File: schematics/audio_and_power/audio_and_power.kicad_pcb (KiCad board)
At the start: 2 copper layers, 85.5 x 88.5 mm, 29 parts, among them J5 Conn_01x03, J6 Conn_01x06, SW1 SW_SPST, SW4 SW_Push, SW5 SW_Push, U2 ESP32-WROOM-32E, U6 MCP4822, U7 PAM8302AAS, U8 LM1117T-3.3

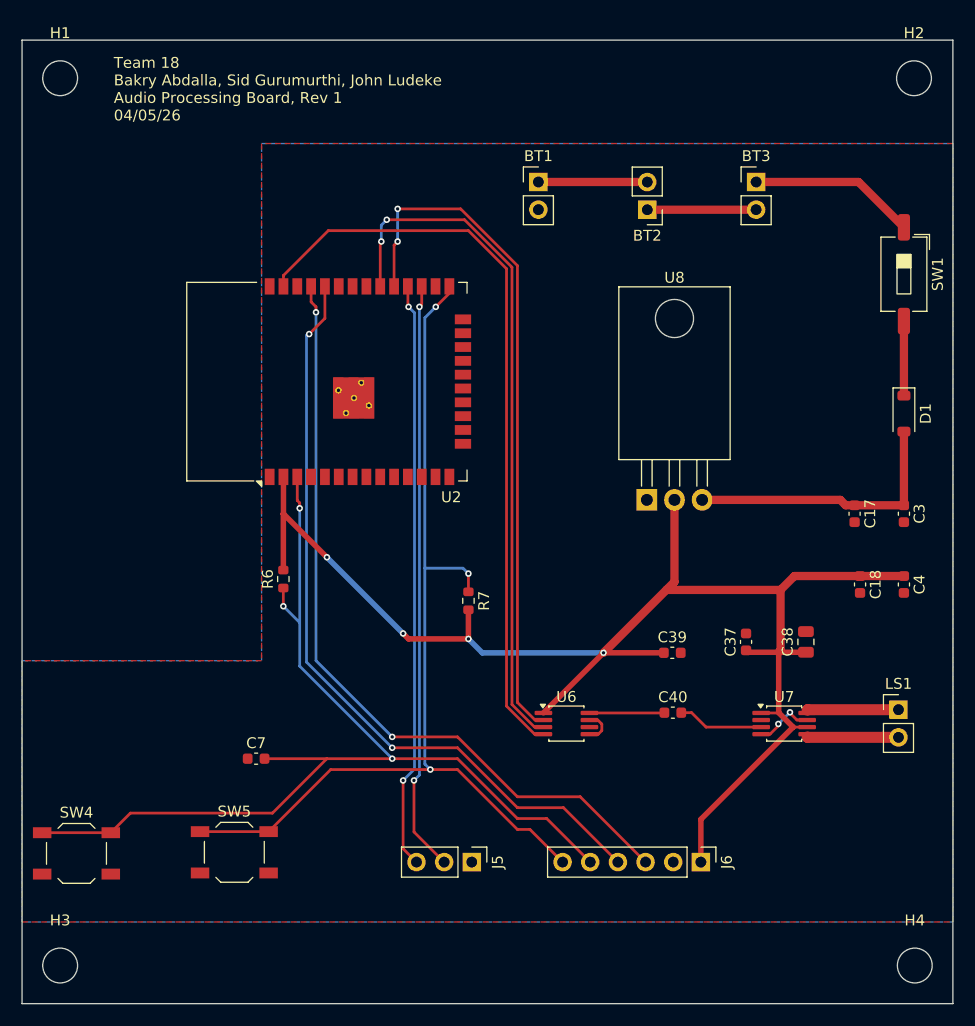
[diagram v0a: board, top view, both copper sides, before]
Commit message: few updates to random things
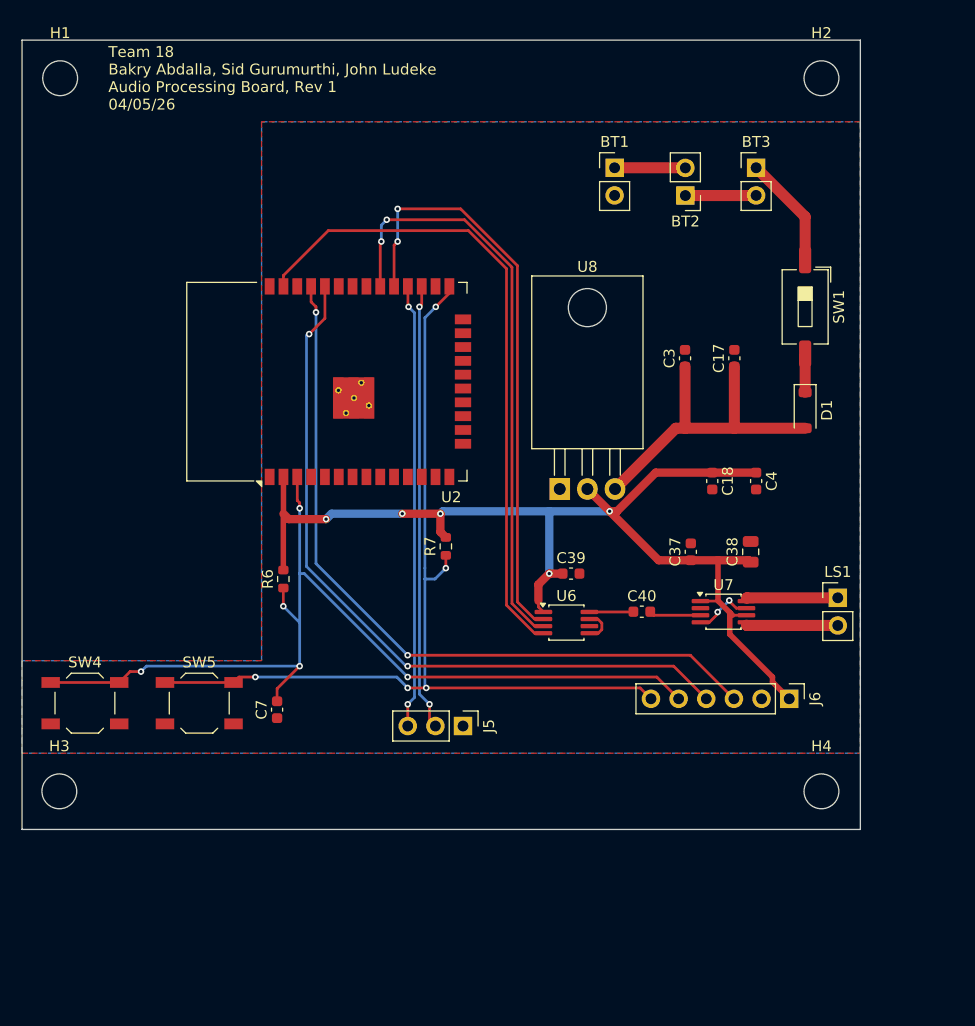
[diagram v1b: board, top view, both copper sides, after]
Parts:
- moved C3 24.7 mm to (107.0, 92.2), turned to 90 degrees
- moved H4 18.2 mm to (119.5, 132.0)
- moved C17 18.0 mm to (111.5, 92.2), turned to 90 degrees
- moved J6 17.1 mm to (116.5, 123.5)
- moved C18 16.6 mm to (109.5, 103.5)
- moved C4 16.6 mm to (113.5, 103.5)
- moved H3 16.0 mm to (49.5, 132.0)
- moved SW5 14.1 mm to (62.4, 123.9)
- moved SW4 13.8 mm to (51.9, 123.9)
- moved J5 12.5 mm to (86.6, 126.0)
- moved C39 11.8 mm to (96.5, 112.0)
- moved LS1 11.7 mm to (121.0, 114.2)
- moved U7 11.7 mm to (110.5, 115.5)
- moved C37 9.71 mm to (107.5, 110.0)
- moved C38 9.71 mm to (113.0, 110.0)
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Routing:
- net /DVDD_3V3: track 136.0 -> 103.9 mm, vias 4 -> 5
- net /TX: track 54.3 -> 41.1 mm
- net /RX: track 54.1 -> 40.9 mm
- net /SCK: track 63.6 -> 54.3 mm
- net /SDI: track 69.3 -> 60.0 mm
- net /CS: track 63.6 -> 54.3 mm
- net /EN: track 96.1 -> 88.4 mm, vias 3 -> 5
- net /VBAT_PROT: track 25.5 -> 31.1 mm
- net /VBAT: track 15.3 -> 10.3 mm
- net Net-(BT2-+): track 10.0 -> 6.50 mm
- net Net-(BT1-+): track 10.0 -> 6.50 mm
- net /IO0: track 90.6 -> 87.1 mm, vias 3 -> 5
- net /TXD0: track 72.5 -> 69.2 mm
- net Net-(D1-K): track 6.85 -> 3.54 mm
- net /RXD0: track 71.5 -> 68.2 mm
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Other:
- board size 85.5 x 88.5 mm -> 77 x 72.5 mm
